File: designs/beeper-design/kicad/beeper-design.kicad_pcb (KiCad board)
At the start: 4 copper layers, 27.5 x 19 mm, 99 parts

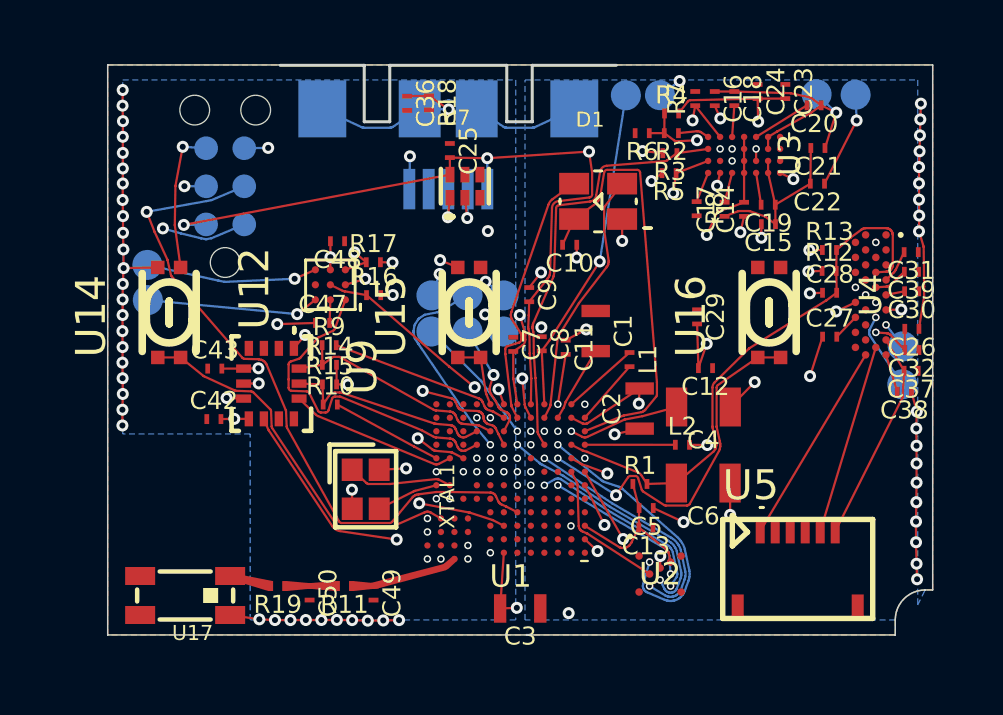
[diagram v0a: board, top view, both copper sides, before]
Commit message: cleaned up kicad export files
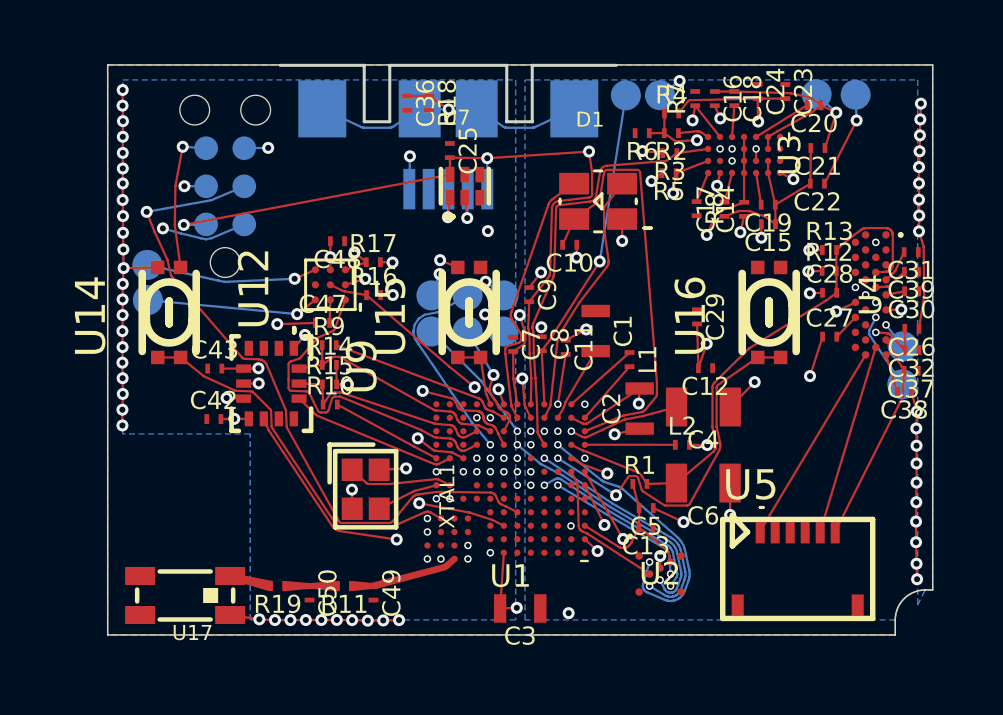
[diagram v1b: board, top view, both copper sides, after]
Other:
- net class BGA removed
- net class Default removed
- net class RF removed
- rule pad_to_mask_clearance: 0.051 -> 0
